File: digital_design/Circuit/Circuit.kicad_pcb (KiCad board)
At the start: 2 copper layers, 100 x 56.1 mm, 36 parts, among them J1 RJ45, J2 RJ45, J3 Conn_01x03_Socket, J4 Conn_01x03_Socket, J5 BAT+, J6 BAT-, Q1 IRF540N, Q2 IRF9540N, U1 PC817, U2 PC817, U3 LM7805_TO220, U4 PC817

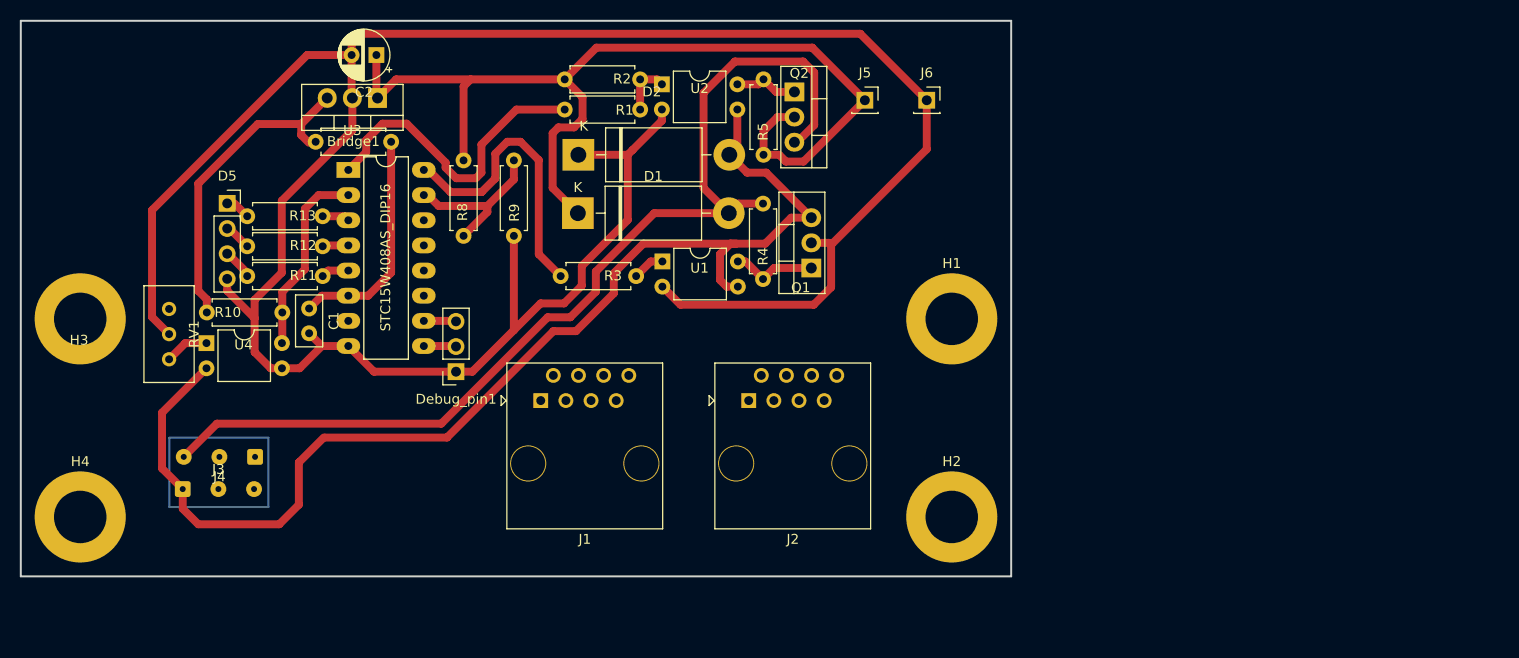
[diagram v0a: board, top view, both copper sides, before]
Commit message: Updated Design as per requirement
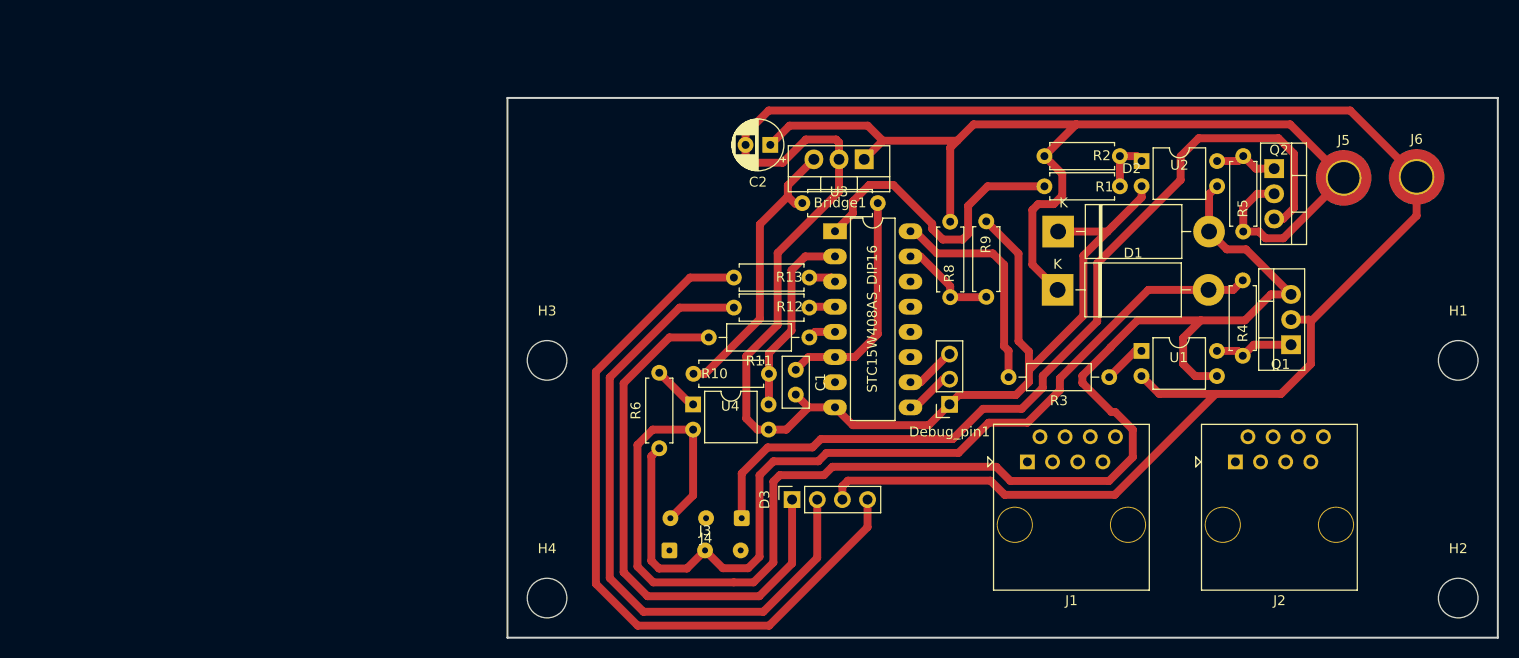
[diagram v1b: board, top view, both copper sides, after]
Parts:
- removed D5: LED_BGRK, Connector_PinSocket_2.54mm:PinSocket_1x04_P2.54mm_Vertical
- removed RV1: 500ohm, Potentiometer_THT:Potentiometer_Bourns_3296W_Vertical
- added D3: LED_BGKR, Connector_PinSocket_2.54mm:PinSocket_1x04_P2.54mm_Vertical, F.Cu at (127.9, 92.2)
- added R6: 180, Resistor_THT:R_Axial_DIN0207_L6.3mm_D2.5mm_P7.62mm_Horizontal, F.Cu at (114.5, 87.1)
- H1, H2, H3, H4: footprint MountingHole:MountingHole_5.3mm_M5_DIN965_Pad -> MountingHole:MountingHole_4mm
- J3, J4: value Conn_01x03_Socket -> 01x03
- J5, J6: footprint Connector_PinSocket_2.54mm:PinSocket_1x01_P2.54mm_Vertical -> MountingHole:MountingHole_3.2mm_M3_DIN965_Pad_TopBottom
- R11, R3: footprint Resistor_THT:R_Axial_DIN0207_L6.3mm_D2.5mm_P7.62mm_Horizontal -> Resistor_THT:R_Axial_DIN0207_L6.3mm_D2.5mm_P10.16mm_Horizontal
- moved H2 51.8 mm to (195.1, 102.2)
- moved H1 51.3 mm to (195.1, 78.2)
- moved J6 50.1 mm to (190.9, 59.7)
- moved Debug_pin1 49.9 mm to (143.8, 82.6)
- moved Bridge1 49.5 mm to (136.5, 62.3)
- moved J1 49.5 mm to (151.6, 88.4)
- moved J2 49.5 mm to (172.6, 88.4)
- moved J4 49.5 mm to (122.8, 94.1)
- moved R10 49.5 mm to (117.9, 79.5)
- moved R8 49.5 mm to (143.8, 71.8)
- moved U3 49.5 mm to (135.2, 57.9)
- moved C1 49.5 mm to (128.2, 79.1)
- moved J3 49.5 mm to (115.5, 97.4)
- moved R11 49.5 mm to (129.6, 75.9)
- moved R12 49.5 mm to (129.6, 72.9)
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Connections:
- J3 pad 1: IN_OUT- -> unconnected-(J3-Pin_1-Pad1)
- J3 pad 2: unconnected-(J3-Pin_2-Pad2) -> IN_OUT+
- J4 pad 1: unconnected-(J4-Pin_1-Pad1) -> BAT_OUT+
- J4 pad 3: IN_OUT+ -> IN_OUT-
- Q2 pad 3: IN_OUT+ -> BAT_OUT+
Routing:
- net BAT_OUT+: track 0.00 -> 88.4 mm
- net Net-(D3-RA): track 1.83 -> 75.4 mm
- net Net-(D3-GA): track 2.53 -> 66.2 mm
- net Net-(D3-BA): track 3.14 -> 55.4 mm
- net IN_OUT-: track 120.0 -> 151.4 mm
- net BAT-: track 261.8 -> 285.8 mm
- net IN_OUT+: track 104.4 -> 90.8 mm
- net BAT+: track 103.0 -> 114.6 mm
- net not NMOS_CONTROL: track 29.5 -> 22.4 mm
- net V_bat_adc: track 16.9 -> 10.3 mm
- net +5V: track 32.2 -> 28.5 mm
- net Net-(Debug_pin1-Pin_2): track 3.27 -> 5.13 mm
- net Net-(Debug_pin1-Pin_3): track 3.27 -> 5.13 mm
- net PMOS_CONTROL: track 31.6 -> 30.3 mm
- net Net-(R3-Pad1): track 3.26 -> 4.36 mm
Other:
- board size 100 x 56.1 mm -> 100 x 54.5 mm
